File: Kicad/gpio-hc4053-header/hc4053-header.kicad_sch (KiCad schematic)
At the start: 6 parts, among them K1 GPIO IN, K3 I/O, K4 I/O, U1 74HC4053, U2 3M-SJ5376

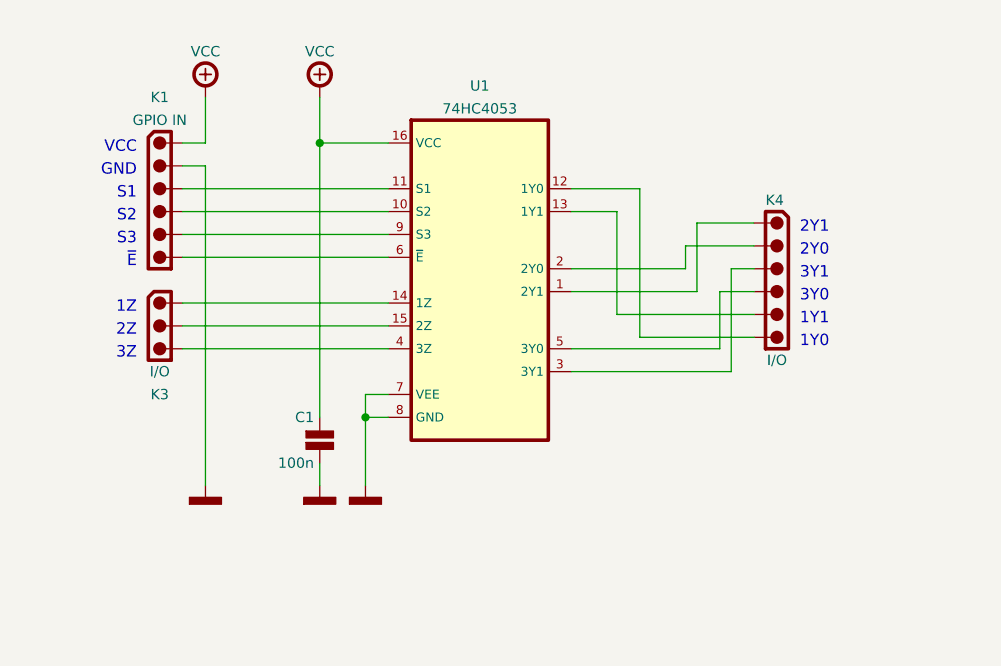
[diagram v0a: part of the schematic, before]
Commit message: Update
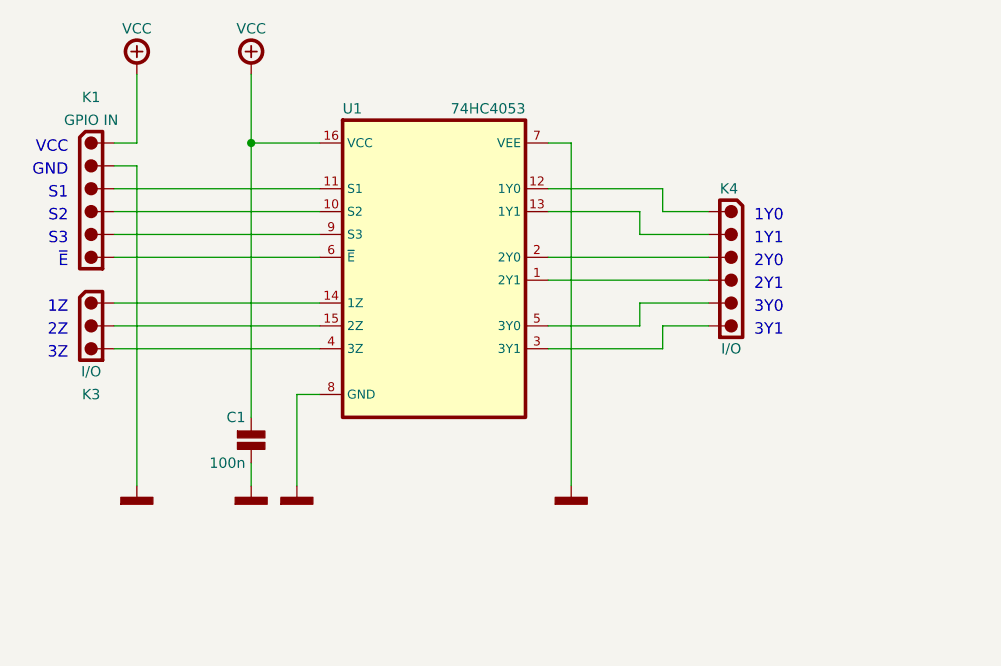
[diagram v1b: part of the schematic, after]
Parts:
- C1: symbol tronixio:C-1206 -> tronixio:CAPACITOR-1206-100N; Mouser (none) -> 80-C1206C104M5R; Name (none) -> CAPACITOR-1206-100N; Tolerance (none) -> 20%; Voltage (none) -> 50V
- K1: Name (none) -> HARWIN-254-M-1X06-RIGHT-ANGLE
- K3: Name (none) -> HARWIN-254-M-1X03-VERTICAL
- K4: Name (none) -> HARWIN-254-M-1X06-VERTICAL
- U1: symbol tronixio:74HC4053 -> tronixio:74HC4053-SOIC-16; Name (none) -> 74HC4053-SOIC-16
- U2: footprint tronixio:zzz3M-SJ5376 -> tronixio:3M-SJ5376
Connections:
- net at K4.1: now also U1.12 (1Y0); no longer U1.1 (2Y1)
- net at K4.2: now also U1.13 (1Y1); no longer U1.2 (2Y0)
- net at K4.3: now also U1.2 (2Y0); no longer U1.3 (3Y1)
- net at K4.4: now also U1.1 (2Y1); no longer U1.5 (3Y0)
- net at K4.5: now also U1.5 (3Y0); no longer U1.13 (1Y1)
- net at K4.6: now also U1.3 (3Y1); no longer U1.12 (1Y0)
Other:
- moved on the sheet: C1, K1, K3, K4, U1
